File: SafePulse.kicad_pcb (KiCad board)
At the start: 4 copper layers, 40.6 x 20.8 mm, 88 parts, among them IC1 S-35770E01I-K8T2U, J1 Conn_01x03_Male, J2 4208, Q1 FQT7N10L, Q2 BC846A, Q3 MMBT3906, Q4 MMBT3906, U1 TS4061AICT-1.25, U2 74HC14, U3 TLV27L1DBVT, U33 MAX9910EXK+T, U4 CD14538BM

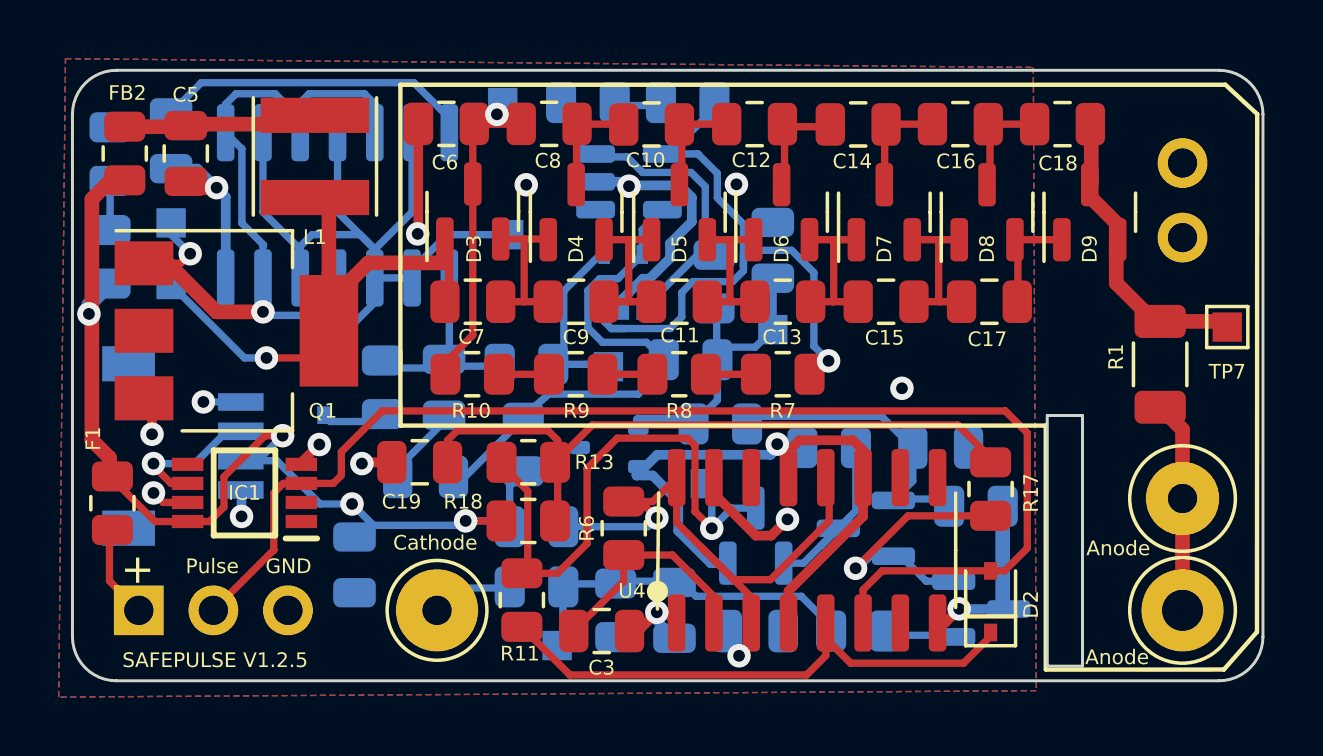
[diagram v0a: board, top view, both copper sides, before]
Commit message: added Allan changes
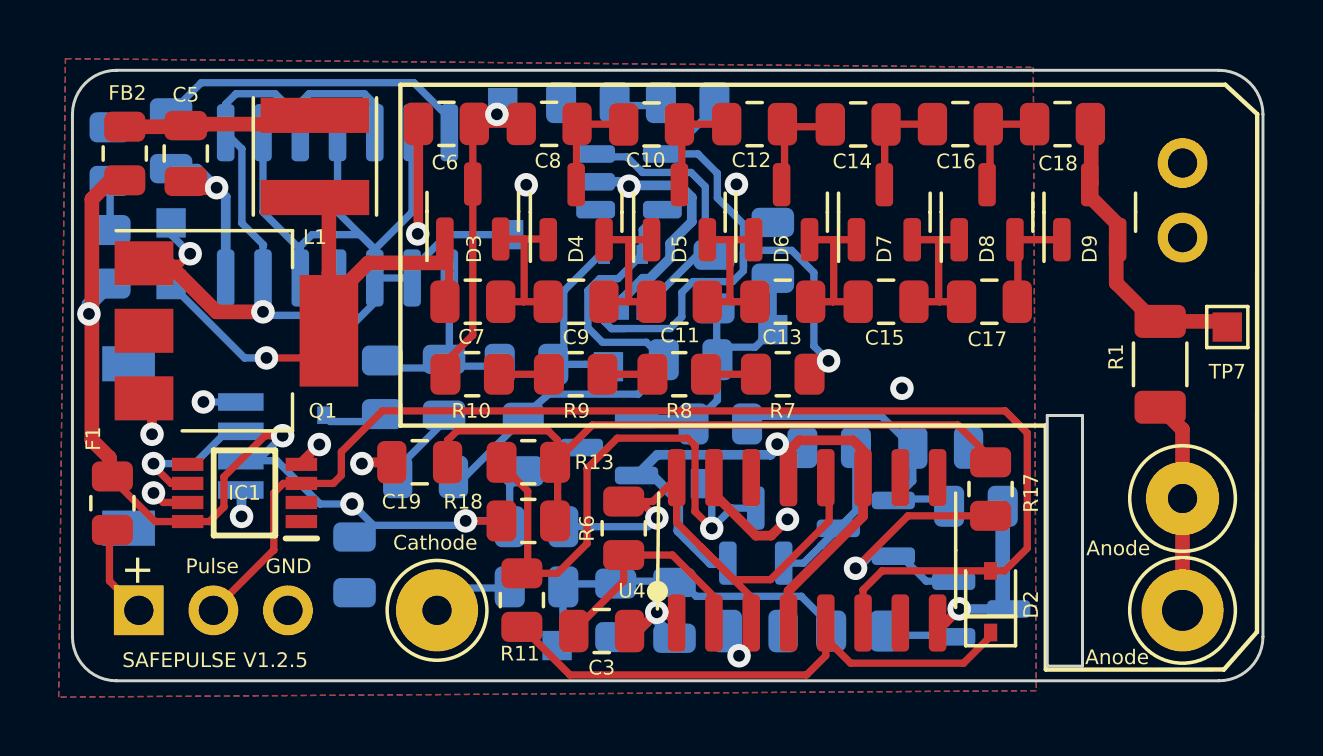
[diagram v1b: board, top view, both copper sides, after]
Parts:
- U1: footprint Package_TO_SOT_SMD:SOT-323_SC-70 -> Package_TO_SOT_SMD:SOT-23
